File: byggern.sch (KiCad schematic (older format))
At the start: 19 parts, among them U1 ATmega162-16PU

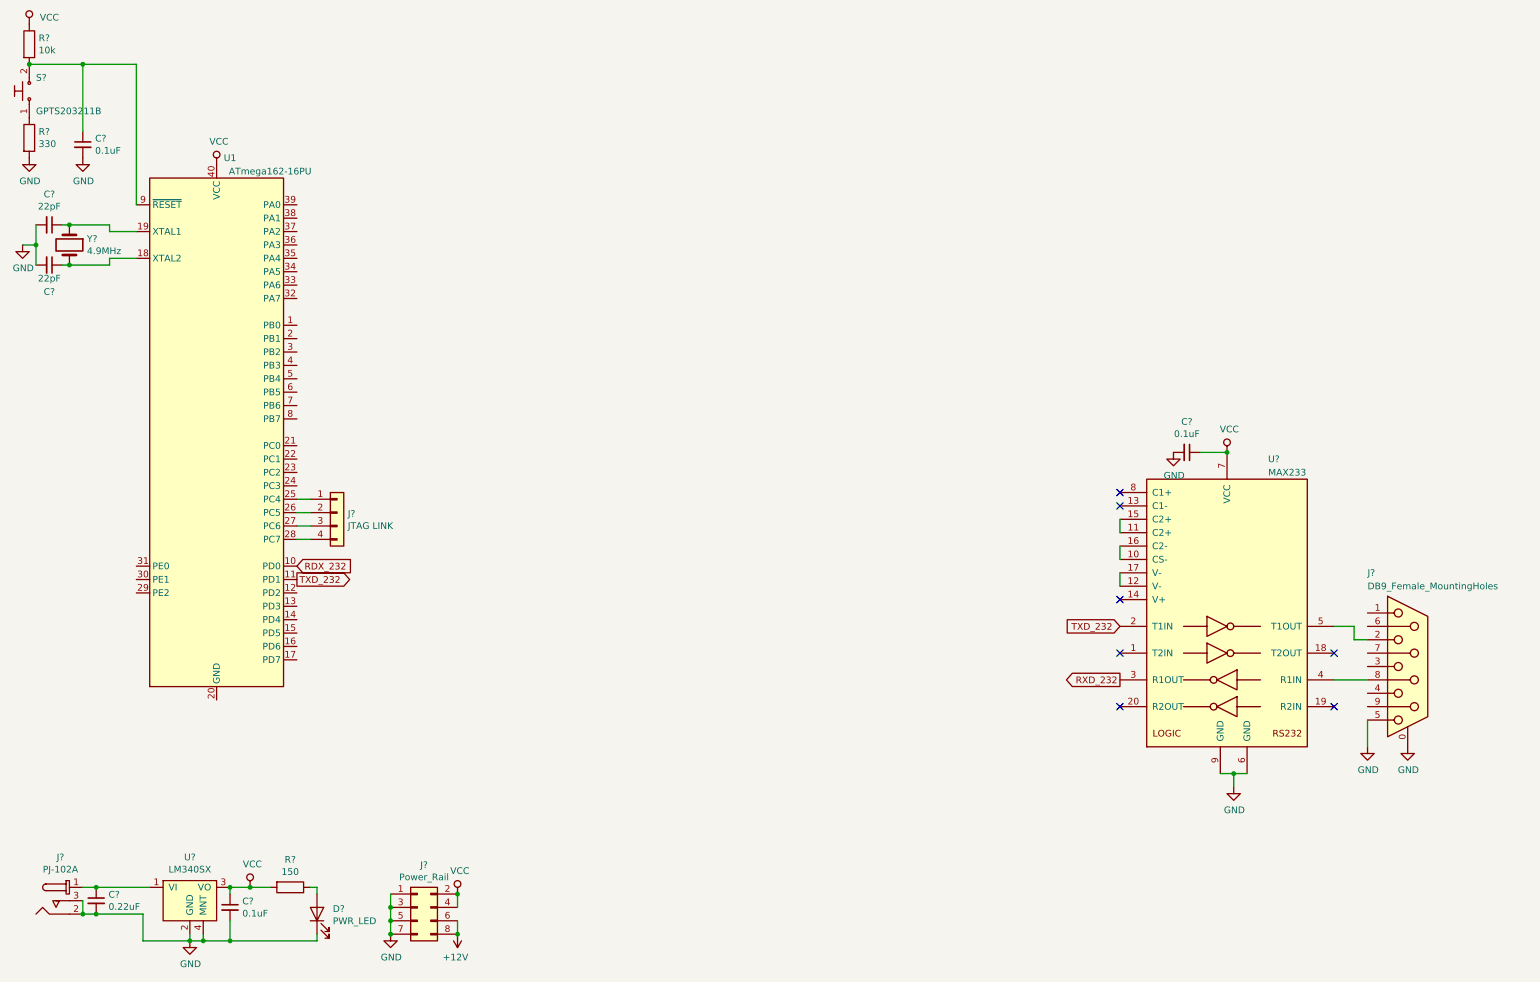
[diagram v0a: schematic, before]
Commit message: Complete schematic, quality check remaining
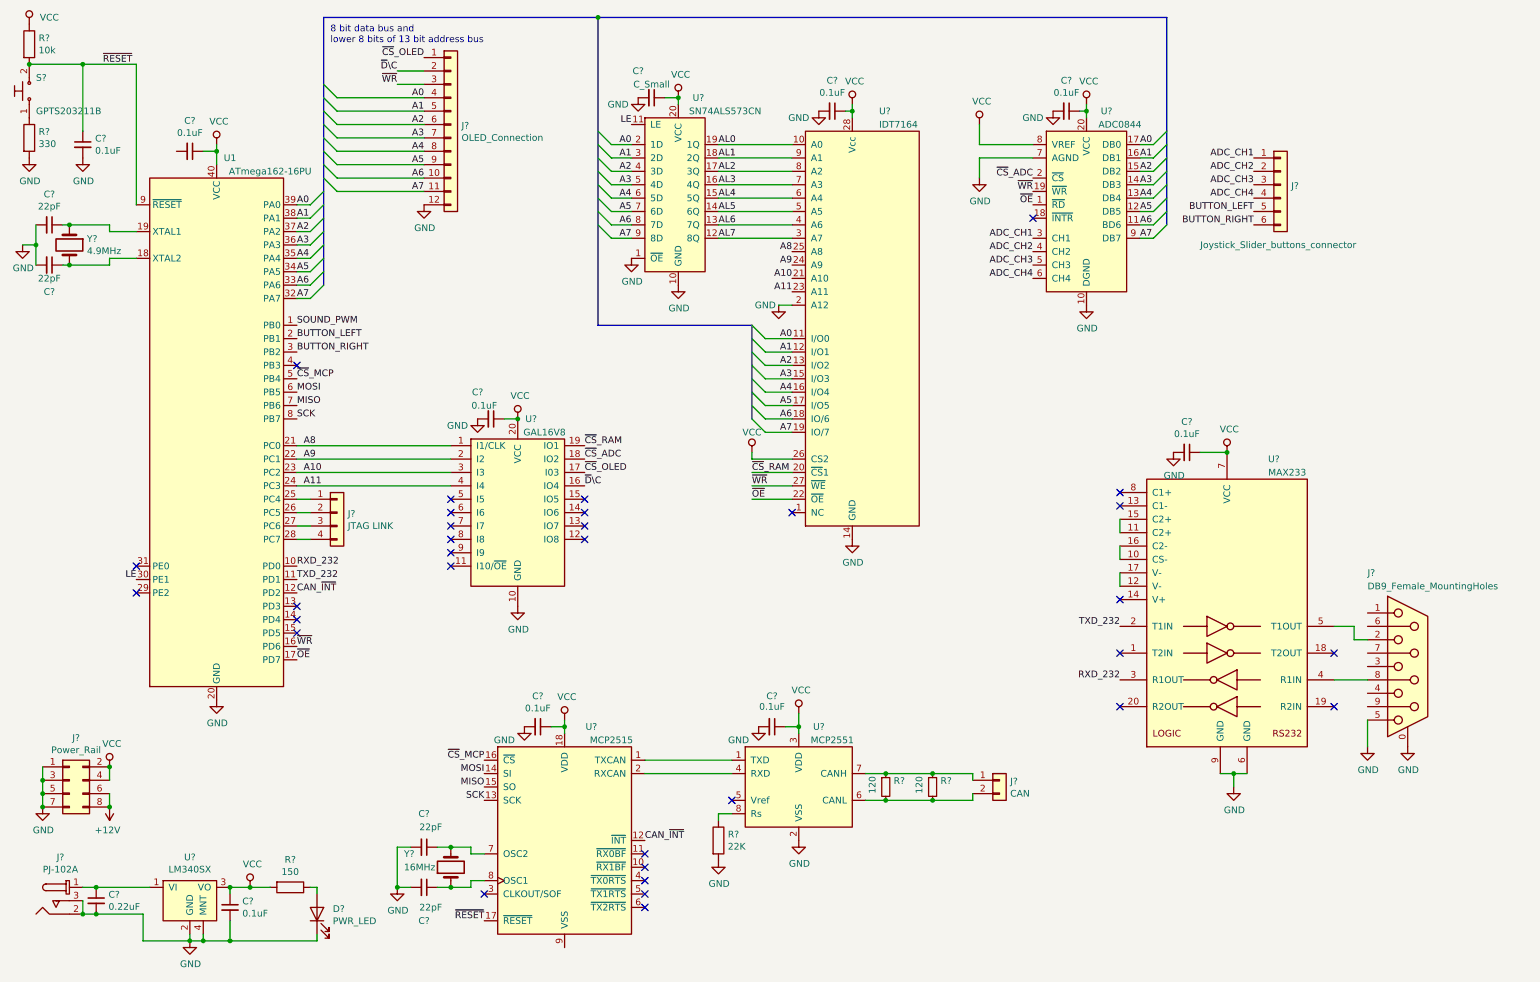
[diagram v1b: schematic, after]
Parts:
- added C? (x6): 0.1uF, symbol Device:C_Small
- added C?: C_Small, symbol Device:C_Small
- added C? (x2): 22pF, symbol Device:C_Small
- added J?: OLED_Connection, symbol Connector_Generic:Conn_01x12
- added J?: Joystick_Slider_buttons_connector, symbol Connector_Generic:Conn_01x06
- added J?: CAN, symbol Connector_Generic:Conn_01x02
- added R?: 22K, symbol Device:R
- added R? (x2): 120, symbol Device:R_Small
- added U?: GAL16V8, symbol Logic_Programmable:GAL16V8
- added U?: SN74ALS573CN, symbol byggern:SN74ALS573CN
- added U?: IDT7164, symbol byggern:IDT7164
- added U?: ADC0844, symbol byggern:ADC0844
- added U?: MCP2515, symbol byggern:MCP2515
- added U?: MCP2551, symbol byggern:MCP2551
- added Y?: 16MHz, symbol Device:Crystal
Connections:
- net RDX_232 is gone; now on net RXD_232: U1.10 (PD0)
- net GND: now also U1.20 (GND), C?.2, C?.2, C?.2, C?.2, C?.2, C?.2, C?.2, C?.2, J?.12 (Pin_12), R?.2, U?.1 (~OE), U?.10 (DGND), U?.10 (GND), U?.10 (GND), U?.14 (GND), U?.2 (A12), U?.2 (VSS), U?.7 (AGND)
- net VCC: now also C?.1, C?.1, C?.1, C?.1, C?.1, C?.1, C?.1, U?.18 (VDD), U?.20 (VCC), U?.20 (VCC), U?.20 (VCC), U?.26 (CS2), U?.28 (Vcc), U?.3 (VDD), U?.8 (VREF)
- net SOUND_PWM: now reaches U1.1 (PB0)
- net CAN_~INT~: now reaches U1.12 (PD2)
- net CAN_~INT~: now also U?.12 (~INT)
- net ~WR~: now reaches U1.16 (PD6)
- net ~WR~: now also J?.3 (Pin_3), U?.19 (~WR), U?.27 (~WE)
- net ~OE~: now reaches U1.17 (PD7)
- net ~OE~: now also U?.1 (~RD), U?.22 (~OE)
- net BUTTON_LEFT: now reaches U1.2 (PB1)
- net BUTTON_LEFT: now also J?.5 (Pin_5)
- net A8: now reaches U1.21 (PC0)
- net A8: now also U?.1 (I1/CLK), U?.25 (A8)
- net A9: now reaches U1.22 (PC1)
- net A9: now also U?.2 (I2), U?.24 (A9)
- net A10: now reaches U1.23 (PC2)
- net A10: now also U?.21 (A10), U?.3 (I3)
- net A11: now reaches U1.24 (PC3)
- net A11: now also U?.23 (A11), U?.4 (I4)
- net BUTTON_RIGHT: now reaches U1.3 (PB2)
- net BUTTON_RIGHT: now also J?.6 (Pin_6)
- net LE: now reaches U1.30 (PE1)
- net LE: now also U?.11 (LE)
- net A7: now reaches U1.32 (PA7)
- net A7: now also J?.11 (Pin_11), U?.19 (IO/7), U?.9 (8D), U?.9 (DB7)
- net A6: now reaches U1.33 (PA6)
- net A6: now also J?.10 (Pin_10), U?.11 (BD6), U?.18 (IO/6), U?.8 (7D)
- net A5: now reaches U1.34 (PA5)
- net A5: now also J?.9 (Pin_9), U?.12 (DB5), U?.17 (I/O5), U?.7 (6D)
- net A4: now reaches U1.35 (PA4)
- net A4: now also J?.8 (Pin_8), U?.13 (DB4), U?.16 (I/O4), U?.6 (5D)
- net A3: now reaches U1.36 (PA3)
- net A3: now also J?.7 (Pin_7), U?.14 (DB3), U?.15 (I/O3), U?.5 (4D)
- net A2: now reaches U1.37 (PA2)
- net A2: now also J?.6 (Pin_6), U?.13 (I/O2), U?.15 (DB2), U?.4 (3D)
- net A1: now reaches U1.38 (PA1)
- net A1: now also J?.5 (Pin_5), U?.12 (I/O1), U?.16 (DB1), U?.3 (2D)
- net A0: now reaches U1.39 (PA0)
- net A0: now also J?.4 (Pin_4), U?.11 (I/O0), U?.17 (DB0), U?.2 (1D)
- net ~CS~_MCP: now reaches U1.5 (PB4)
- net ~CS~_MCP: now also U?.16 (~CS)
- net MOSI: now reaches U1.6 (PB5)
- net MOSI: now also U?.14 (SI)
- net MISO: now reaches U1.7 (PB6)
- net MISO: now also U?.15 (SO)
- net SCK: now reaches U1.8 (PB7)
- net SCK: now also U?.13 (SCK)
- net ~RESET~: now reaches C?.1, R?.2, S?.2, U1.9 (~RESET)
- net ~RESET~: now also U?.17 (~RESET)
- new net: U?.1 (TXCAN), U?.1 (TXD)
- new net: U?.2 (RXCAN), U?.4 (RXD)
- new net: C?.1, U?.7 (OSC2), Y?.2
- new net: C?.1, U?.8 (OSC1), Y?.1
- new net: J?.2 (Pin_2), R?.2, R?.2, U?.6 (CANL)
- new net: J?.1 (Pin_1), R?.1, R?.1, U?.7 (CANH)
- new net: R?.1, U?.8 (Rs)
- new net ADC_CH1: J?.1 (Pin_1), U?.3 (CH1)
- new net ADC_CH2: J?.2 (Pin_2), U?.4 (CH2)
- new net ADC_CH3: J?.3 (Pin_3), U?.5 (CH3)
- new net ADC_CH4: J?.4 (Pin_4), U?.6 (CH4)
- new net AL0: U?.10 (A0), U?.19 (1Q)
- new net AL1: U?.18 (2Q), U?.9 (A1)
- new net AL2: U?.17 (3Q), U?.8 (A2)
- new net AL3: U?.16 (4Q), U?.7 (A3)
- new net AL4: U?.15 (5Q), U?.6 (A4)
- new net AL5: U?.14 (6Q), U?.5 (A5)
- new net AL6: U?.13 (7Q), U?.4 (A6)
- new net AL7: U?.12 (8Q), U?.3 (A7)
- new net ~CS~_ADC: U?.18 (IO2), U?.2 (~CS~)
- new net ~CS~_OLED: J?.1 (Pin_1), U?.17 (I03)
- new net ~CS~_RAM: U?.19 (IO1), U?.20 (~CS~1)
- new net ~D~\C: J?.2 (Pin_2), U?.16 (IO4)
- no-connect marks 7 -> 32
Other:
- note added: "8 bit data bus and\nlower 8 bits of 13 bit address bus"
- moved on the sheet: J?
